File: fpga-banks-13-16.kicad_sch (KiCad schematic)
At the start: 48 parts, among them U14 XC7A100T-FGG484, U15 Oscillator_100MHz_AMJMEFB

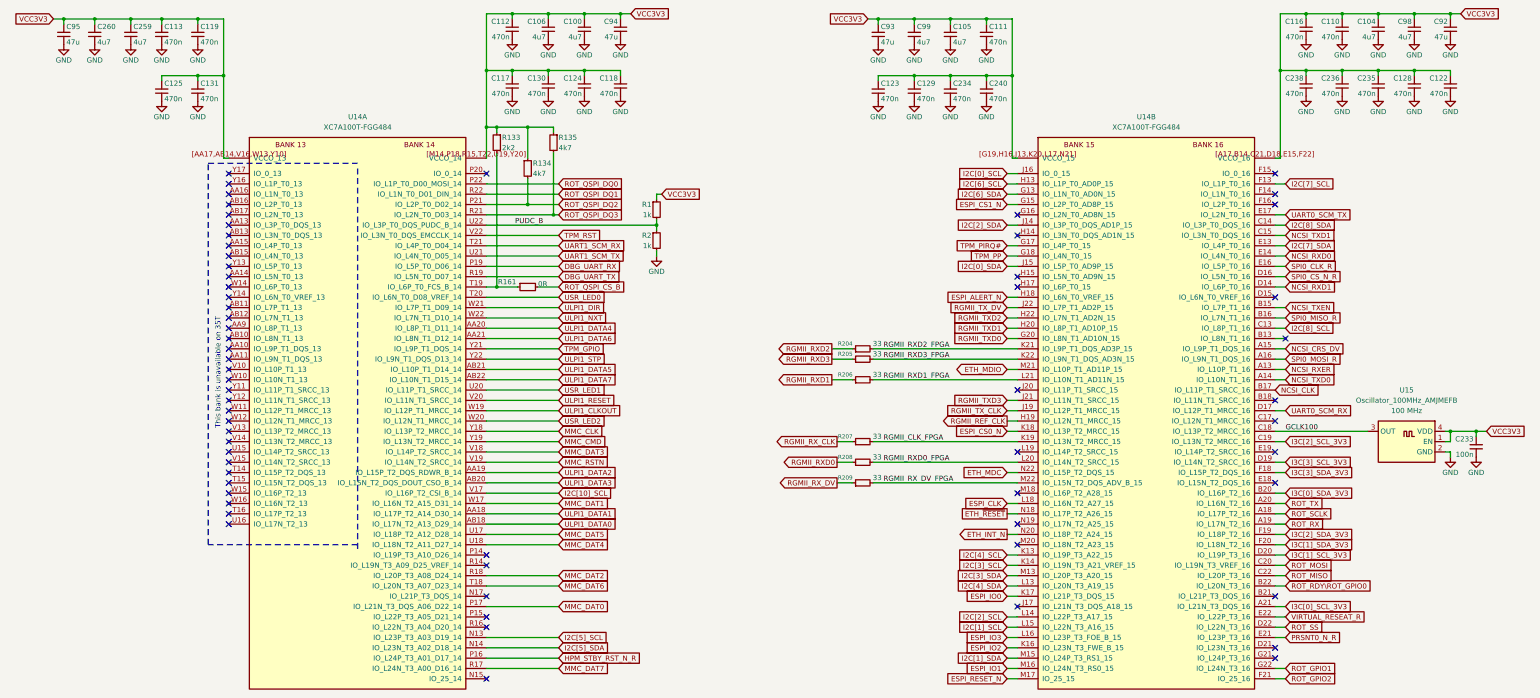
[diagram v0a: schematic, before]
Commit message: river routing
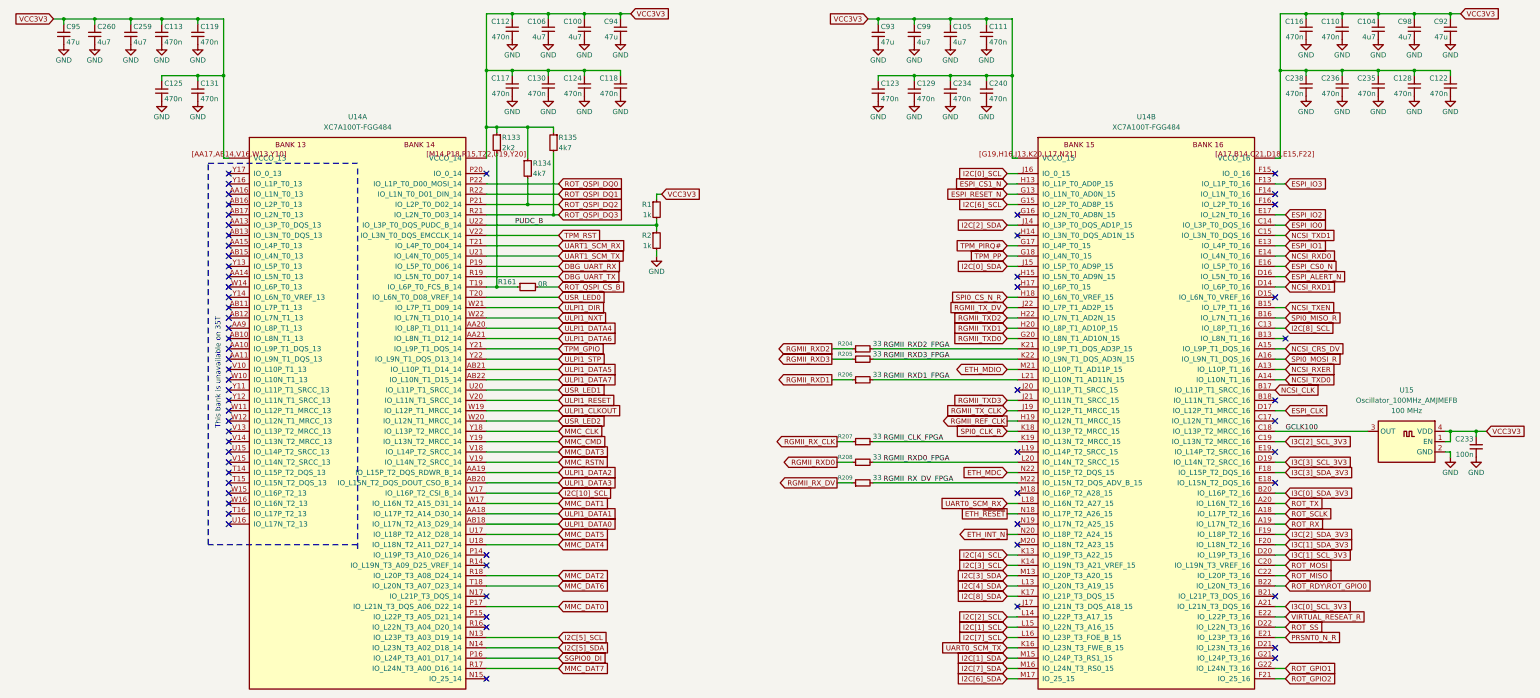
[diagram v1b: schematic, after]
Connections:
- net ESPI_ALERT_N: now also U14.D16 (IO_L5N_T0_16); no longer U14.H18 (IO_L6N_T0_VREF_15)
- net ESPI_CLK: now also U14.D17 (IO_L12P_T1_MRCC_16); no longer U14.L18 (IO_L16N_T2_A27_15)
- net ESPI_CS0_N: now also U14.E16 (IO_L5P_T0_16); no longer U14.K18 (IO_L13P_T2_MRCC_15)
- net ESPI_CS1_N: now also U14.H13 (IO_L1P_T0_AD0P_15); no longer U14.G15 (IO_L2P_T0_AD8P_15)
- net ESPI_IO0: now also U14.C14 (IO_L3P_T0_DQS_16); no longer U14.K17 (IO_L21P_T3_DQS_15)
- net ESPI_IO1: now also U14.E13 (IO_L4P_T0_16); no longer U14.M16 (IO_L24N_T3_RS0_15)
- net ESPI_IO2: now also U14.E17 (IO_L2N_T0_16); no longer U14.K16 (IO_L23N_T3_FWE_B_15)
- net ESPI_IO3: now also U14.F13 (IO_L1P_T0_16); no longer U14.L16 (IO_L23P_T3_FOE_B_15)
- net ESPI_RESET_N: now also U14.G13 (IO_L1N_T0_AD0N_15); no longer U14.M17 (IO_25_15)
- net I2C[6]_SCL: now also U14.G15 (IO_L2P_T0_AD8P_15); no longer U14.H13 (IO_L1P_T0_AD0P_15)
- net I2C[6]_SDA: now also U14.M17 (IO_25_15); no longer U14.G13 (IO_L1N_T0_AD0N_15)
- net I2C[7]_SCL: now also U14.L16 (IO_L23P_T3_FOE_B_15); no longer U14.F13 (IO_L1P_T0_16)
- net I2C[7]_SDA: now also U14.M16 (IO_L24N_T3_RS0_15); no longer U14.E13 (IO_L4P_T0_16)
- net I2C[8]_SDA: now also U14.K17 (IO_L21P_T3_DQS_15); no longer U14.C14 (IO_L3P_T0_DQS_16)
- net SPI0_CLK_R: now also U14.K18 (IO_L13P_T2_MRCC_15); no longer U14.E16 (IO_L5P_T0_16)
- net SPI0_CS_N_R: now also U14.H18 (IO_L6N_T0_VREF_15); no longer U14.D16 (IO_L5N_T0_16)
- net UART0_SCM_RX: now also U14.L18 (IO_L16N_T2_A27_15); no longer U14.D17 (IO_L12P_T1_MRCC_16)
- net UART0_SCM_TX: now also U14.K16 (IO_L23N_T3_FWE_B_15); no longer U14.E17 (IO_L2N_T0_16)
- net HPM_STBY_RST_N_R renamed SGPIO0_DI

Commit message: Almost done with the routing
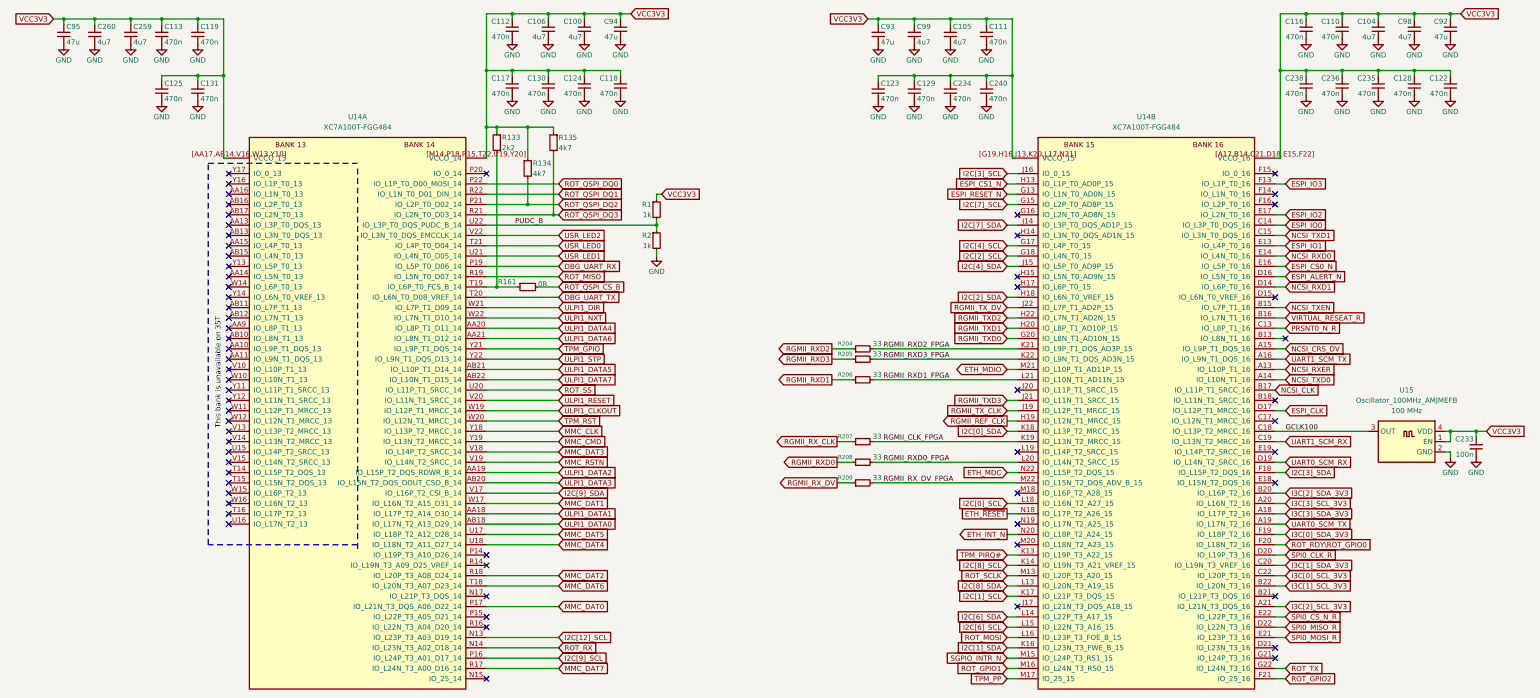
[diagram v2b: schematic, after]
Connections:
- net I2C[5]_SDA is gone; now on net ROT_RX: U14.N14 (IO_L23N_T3_A02_D18_14)
- net DBG_UART_TX: now also U14.T20 (IO_L6N_T0_D08_VREF_14); no longer U14.R19 (IO_L5N_T0_D07_14)
- net I2C[0]_SCL: now also U14.L18 (IO_L16N_T2_A27_15); no longer U14.J16 (IO_0_15)
- net I2C[0]_SDA: now also U14.K18 (IO_L13P_T2_MRCC_15); no longer U14.J15 (IO_L5P_T0_AD9P_15)
- net I2C[1]_SCL: now also U14.K17 (IO_L21P_T3_DQS_15); no longer U14.L15 (IO_L22N_T3_A16_15)
- net I2C[1]_SDA: now also U14.K16 (IO_L23N_T3_FWE_B_15); no longer U14.M15 (IO_L24P_T3_RS1_15)
- net I2C[2]_SCL: now also U14.G18 (IO_L4N_T0_15); no longer U14.L14 (IO_L22P_T3_A17_15)
- net I2C[2]_SDA: now also U14.H18 (IO_L6N_T0_VREF_15); no longer U14.J14 (IO_L3P_T0_DQS_AD1P_15)
- net I2C[3]_SCL: now also U14.J16 (IO_0_15); no longer U14.K14 (IO_L19N_T3_A21_VREF_15)
- net I2C[3]_SDA: now also U14.F18 (IO_L15P_T2_DQS_16); no longer U14.M13 (IO_L20P_T3_A20_15)
- net I2C[4]_SCL: now also U14.G17 (IO_L4P_T0_15); no longer U14.K13 (IO_L19P_T3_A22_15)
- net I2C[4]_SDA: now also U14.J15 (IO_L5P_T0_AD9P_15); no longer U14.L13 (IO_L20N_T3_A19_15)
- net I2C[6]_SCL: now also U14.L15 (IO_L22N_T3_A16_15); no longer U14.G15 (IO_L2P_T0_AD8P_15)
- net I2C[6]_SDA: now also U14.L14 (IO_L22P_T3_A17_15); no longer U14.M17 (IO_25_15)
- net I2C[7]_SCL: now also U14.G15 (IO_L2P_T0_AD8P_15); no longer U14.L16 (IO_L23P_T3_FOE_B_15)
- net I2C[7]_SDA: now also U14.J14 (IO_L3P_T0_DQS_AD1P_15); no longer U14.M16 (IO_L24N_T3_RS0_15)
- net I2C[8]_SCL: now also U14.K14 (IO_L19N_T3_A21_VREF_15); no longer U14.C13 (IO_L8P_T1_16)
- net I2C[8]_SDA: now also U14.L13 (IO_L20N_T3_A19_15); no longer U14.K17 (IO_L21P_T3_DQS_15)
- net I3C[0]_SCL_3V3: now also U14.C22 (IO_L20P_T3_16); no longer U14.A21 (IO_L21N_T3_DQS_16)
- net I3C[0]_SDA_3V3: now also U14.F19 (IO_L18P_T2_16); no longer U14.B20 (IO_L16P_T2_16)
- net I3C[1]_SCL_3V3: now also U14.B22 (IO_L20N_T3_16); no longer U14.D20 (IO_L19P_T3_16)
- net I3C[1]_SDA_3V3: now also U14.C20 (IO_L19N_T3_VREF_16); no longer U14.F20 (IO_L18N_T2_16)
- net I3C[2]_SCL_3V3: now also U14.A21 (IO_L21N_T3_DQS_16); no longer U14.C19 (IO_L13N_T2_MRCC_16)
- net I3C[2]_SDA_3V3: now also U14.B20 (IO_L16P_T2_16); no longer U14.F19 (IO_L18P_T2_16)
- net I3C[3]_SCL_3V3: now also U14.A20 (IO_L16N_T2_16); no longer U14.D19 (IO_L14N_T2_SRCC_16)
- net I3C[3]_SDA_3V3: now also U14.A18 (IO_L17P_T2_16); no longer U14.F18 (IO_L15P_T2_DQS_16)
- net PRSNT0_N_R: now also U14.C13 (IO_L8P_T1_16); no longer U14.E21 (IO_L23P_T3_16)
- net ROT_GPIO1: now also U14.M16 (IO_L24N_T3_RS0_15); no longer U14.G22 (IO_L24N_T3_16)
- net ROT_MISO: now also U14.R19 (IO_L5N_T0_D07_14); no longer U14.C22 (IO_L20P_T3_16)
- net ROT_MOSI: now also U14.L16 (IO_L23P_T3_FOE_B_15); no longer U14.C20 (IO_L19N_T3_VREF_16)
- net ROT_RDY\ROT_GPIO0: now also U14.F20 (IO_L18N_T2_16); no longer U14.B22 (IO_L20N_T3_16)
- net ROT_RX: no longer U14.A19 (IO_L17N_T2_16)
- net ROT_SCLK: now also U14.M13 (IO_L20P_T3_A20_15); no longer U14.A18 (IO_L17P_T2_16)
- net ROT_SS: now also U14.U20 (IO_L11P_T1_SRCC_14); no longer U14.D22 (IO_L22N_T3_16)
- net ROT_TX: now also U14.G22 (IO_L24N_T3_16); no longer U14.A20 (IO_L16N_T2_16)
- net SPI0_CLK_R: now also U14.D20 (IO_L19P_T3_16); no longer U14.K18 (IO_L13P_T2_MRCC_15)
- net SPI0_CS_N_R: now also U14.E22 (IO_L22P_T3_16); no longer U14.H18 (IO_L6N_T0_VREF_15)
- net SPI0_MISO_R: now also U14.D22 (IO_L22N_T3_16); no longer U14.B16 (IO_L7N_T1_16)
- net SPI0_MOSI_R: now also U14.E21 (IO_L23P_T3_16); no longer U14.A16 (IO_L9N_T1_DQS_16)
- net TPM_PIRQ#: now also U14.K13 (IO_L19P_T3_A22_15); no longer U14.G17 (IO_L4P_T0_15)
- net TPM_PP: now also U14.M17 (IO_25_15); no longer U14.G18 (IO_L4N_T0_15)
- net TPM_RST: now also U14.W20 (IO_L12N_T1_MRCC_14); no longer U14.V22 (IO_L3N_T0_DQS_EMCCLK_14)
- net UART0_SCM_RX: now also U14.D19 (IO_L14N_T2_SRCC_16); no longer U14.L18 (IO_L16N_T2_A27_15)
- net UART0_SCM_TX: now also U14.A19 (IO_L17N_T2_16); no longer U14.K16 (IO_L23N_T3_FWE_B_15)
- net UART1_SCM_RX: now also U14.C19 (IO_L13N_T2_MRCC_16); no longer U14.T21 (IO_L4P_T0_D04_14)
- net UART1_SCM_TX: now also U14.A16 (IO_L9N_T1_DQS_16); no longer U14.U21 (IO_L4N_T0_D05_14)
- net USR_LED0: now also U14.T21 (IO_L4P_T0_D04_14); no longer U14.T20 (IO_L6N_T0_D08_VREF_14)
- net USR_LED1: now also U14.U21 (IO_L4N_T0_D05_14); no longer U14.U20 (IO_L11P_T1_SRCC_14)
- net USR_LED2: now also U14.V22 (IO_L3N_T0_DQS_EMCCLK_14); no longer U14.W20 (IO_L12N_T1_MRCC_14)
- net VIRTUAL_RESEAT_R: now also U14.B16 (IO_L7N_T1_16); no longer U14.E22 (IO_L22P_T3_16)
- net I2C[10]_SCL renamed I2C[9]_SDA
- net I2C[5]_SCL renamed I2C[12]_SCL
- net SGPIO0_DI renamed I2C[9]_SCL
- new net SGPIO_INTR_N: U14.M15 (IO_L24P_T3_RS1_15)
